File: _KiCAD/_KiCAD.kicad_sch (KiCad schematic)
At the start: 3 parts, among them J1 RJ45, U1 ESP32-WROOM-32

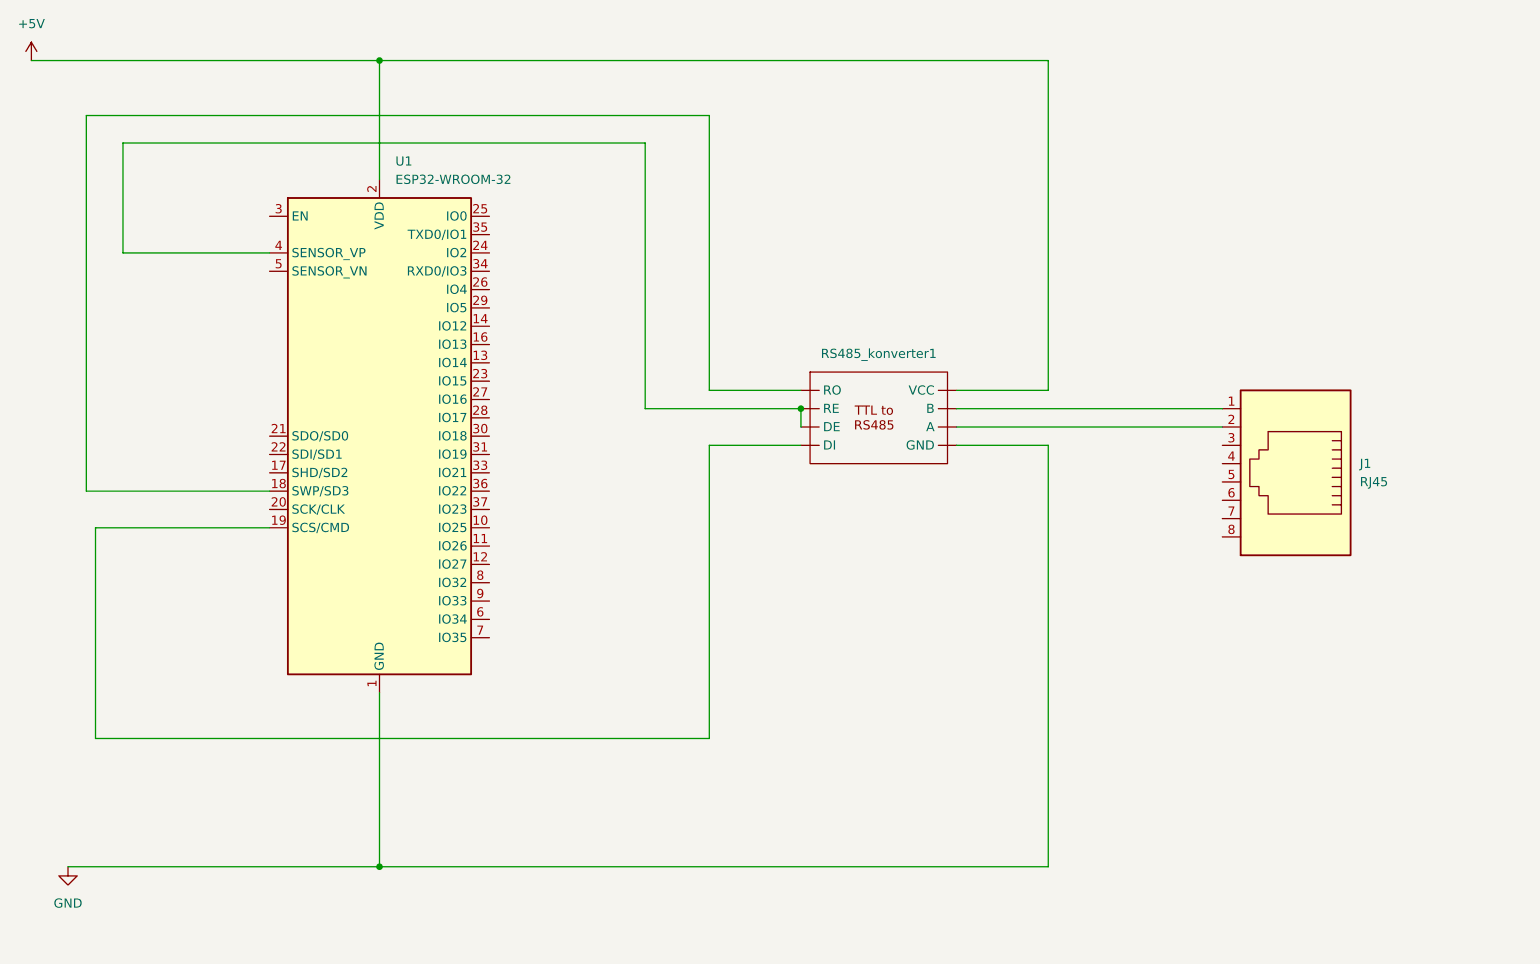
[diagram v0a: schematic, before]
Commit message: new
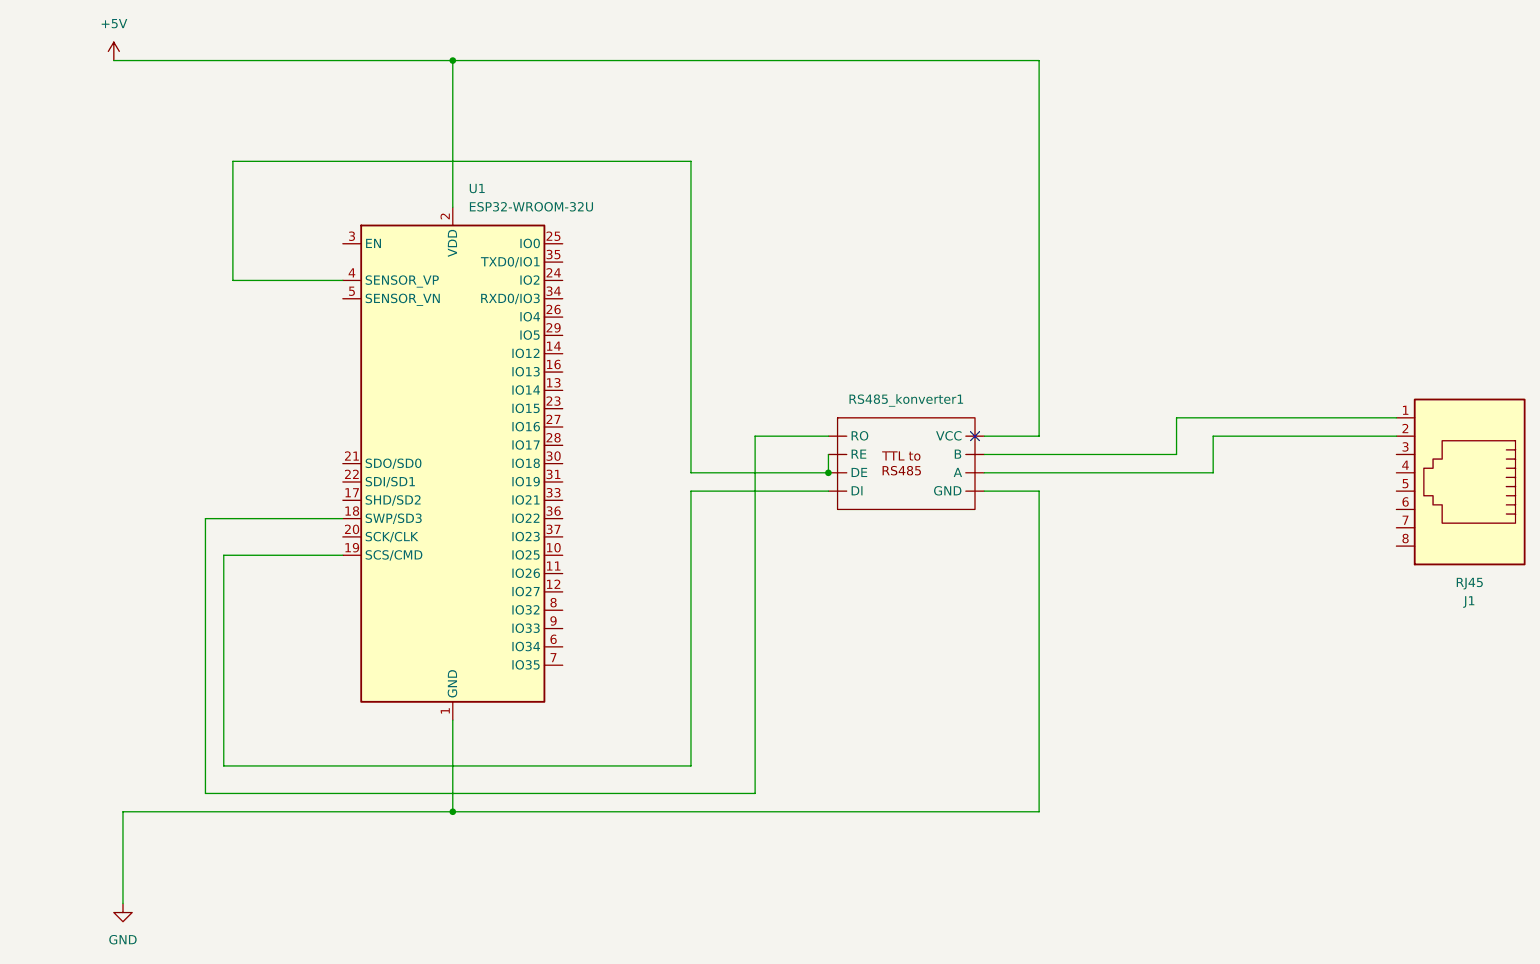
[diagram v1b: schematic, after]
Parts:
- removed U1: ESP32-WROOM-32, RF_Module:ESP32-WROOM-32, symbol RF_Module:ESP32-WROOM-32
- added U1: ESP32-WROOM-32U, RF_Module:ESP32-WROOM-32U, symbol RF_Module:ESP32-WROOM-32U
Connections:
- net +5V: now also U1.2 (VDD)
- net GND: now also U1.1 (GND), U1.15 (GND), U1.38 (GND), U1.39 (GND)
- new net: RS485_konverter1. (VCC), U1.18 (SWP/SD3)
- new net: RS485_konverter1. (VCC), U1.19 (SCS/CMD)
- new net: RS485_konverter1. (VCC), U1.4 (SENSOR_VP)
- no-connect marks 0 -> 1
